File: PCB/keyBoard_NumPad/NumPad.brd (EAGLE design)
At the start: 88.9 x 142.9 mm, 174 parts, among them J1 J, J10 J, J11 J, J12 J, J13 J, J14 J, J15 J, J16 J, J17 J, J2 J, J3 J, J4 J, J5 J, J6 J, J7 J, J8 J, J9 J

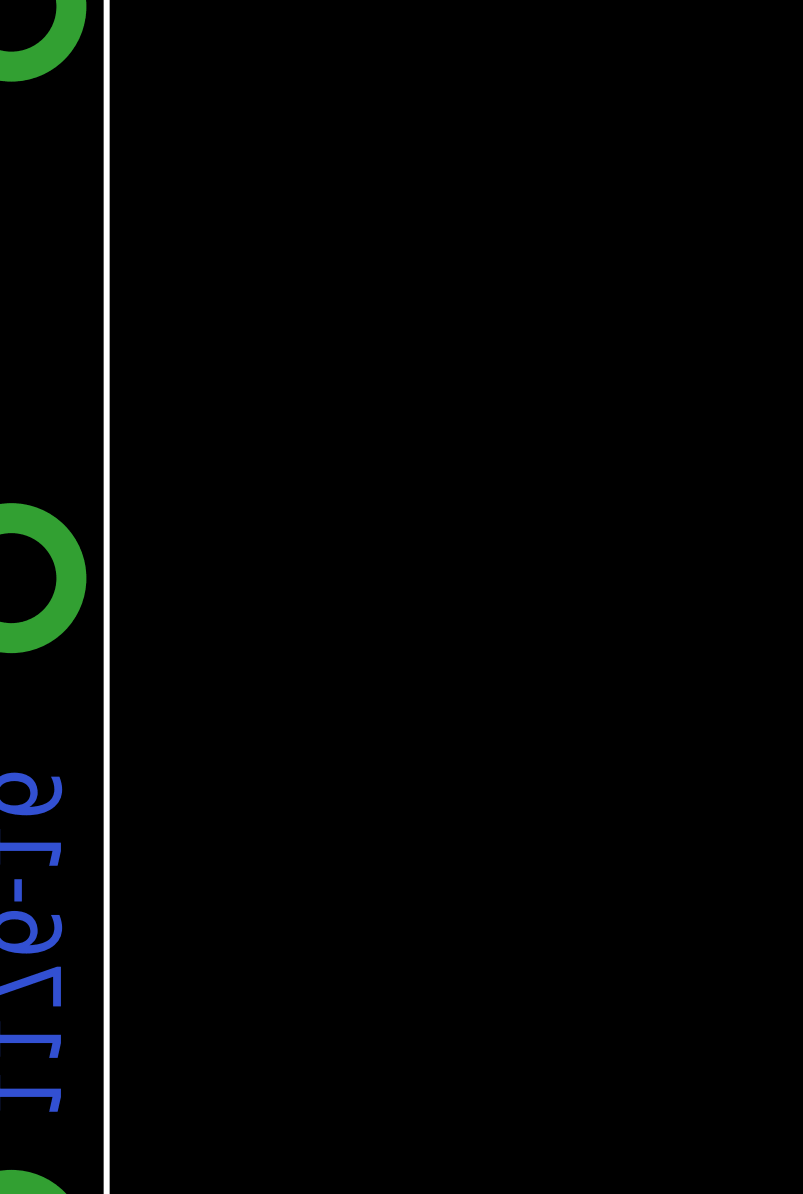
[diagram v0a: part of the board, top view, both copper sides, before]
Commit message: add1
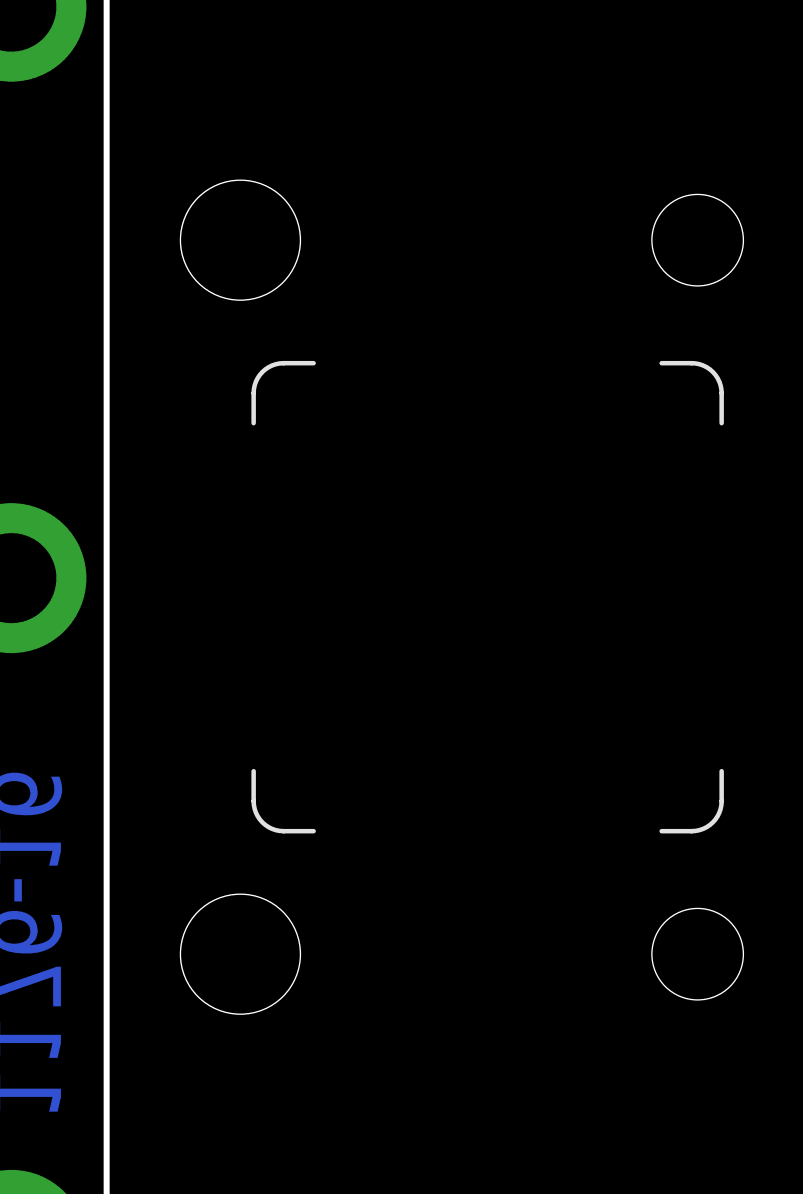
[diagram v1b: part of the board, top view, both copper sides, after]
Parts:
- added STAB_NEN: STAB, kbmxco:ZEALIOS-PCB_2U
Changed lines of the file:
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@@
 <?xml version="1.0" encoding="utf-8"?>
 <!DOCTYPE eagle SYSTEM "eagle.dtd">
-<eagle version="6.3">
+<eagle version="6.4">
 <drawing>
 <settings>
@@
 <circle x="43.4975" y="115.57" radius="3" width="0.254" layer="20"/>
 <circle x="62.5475" y="77.47" radius="3" width="0.254" layer="20"/>
-<dimension x1="18.0975" y1="156.36875" x2="106.9975" y2="154.94" x3="62.5475" y3="159.86125" layer="130" dtype="horizontal"/>
-<dimension x1="107.6325" y1="156.845" x2="106.68" y2="13.97" x3="117.7925" y3="85.4075" layer="130" dtype="vertical"/>
+<dimension x1="18.0975" y1="156.36875" x2="106.9975" y2="154.94" x3="62.5475" y3="159.86125" textsize="3.5" layer="130" dtype="horizontal"/>
+<dimension x1="107.6325" y1="156.845" x2="106.68" y2="13.97" x3="117.7925" y3="85.4075" textsize="3.5" layer="130" dtype="vertical"/>
 <wire x1="103.8225" y1="156.845" x2="21.2725" y2="156.845" width="0.2" layer="20"/>
-<dimension x1="108.74375" y1="115.57" x2="108.42625" y2="96.52" x3="113.82375" y3="106.045" layer="130" dtype="vertical"/>
+<dimension x1="108.74375" y1="115.57" x2="108.42625" y2="96.52" x3="113.82375" y3="106.045" textsize="3.5" layer="130" dtype="vertical"/>
 <wire x1="106.9975" y1="153.67" x2="106.9975" y2="17.145" width="0.2" layer="20"/>
 <wire x1="106.9975" y1="17.145" x2="103.8225" y2="13.97" width="0.2" layer="20" curve="-90"/>
@@
 <element name="U$24" library="kbmxco" package="KEY" value="" x="36.5125" y="125.095"/>
 <element name="U$26" library="kbmxco" package="SIZE132" value="" x="13.0175" y="88.5825"/>
+<element name="STAB_NEN" library="kbmxco" package="ZEALIOS-PCB_2U" value="STAB" x="119.6975" y="38.735" rot="R270"/>
 </elements>
 <signals>

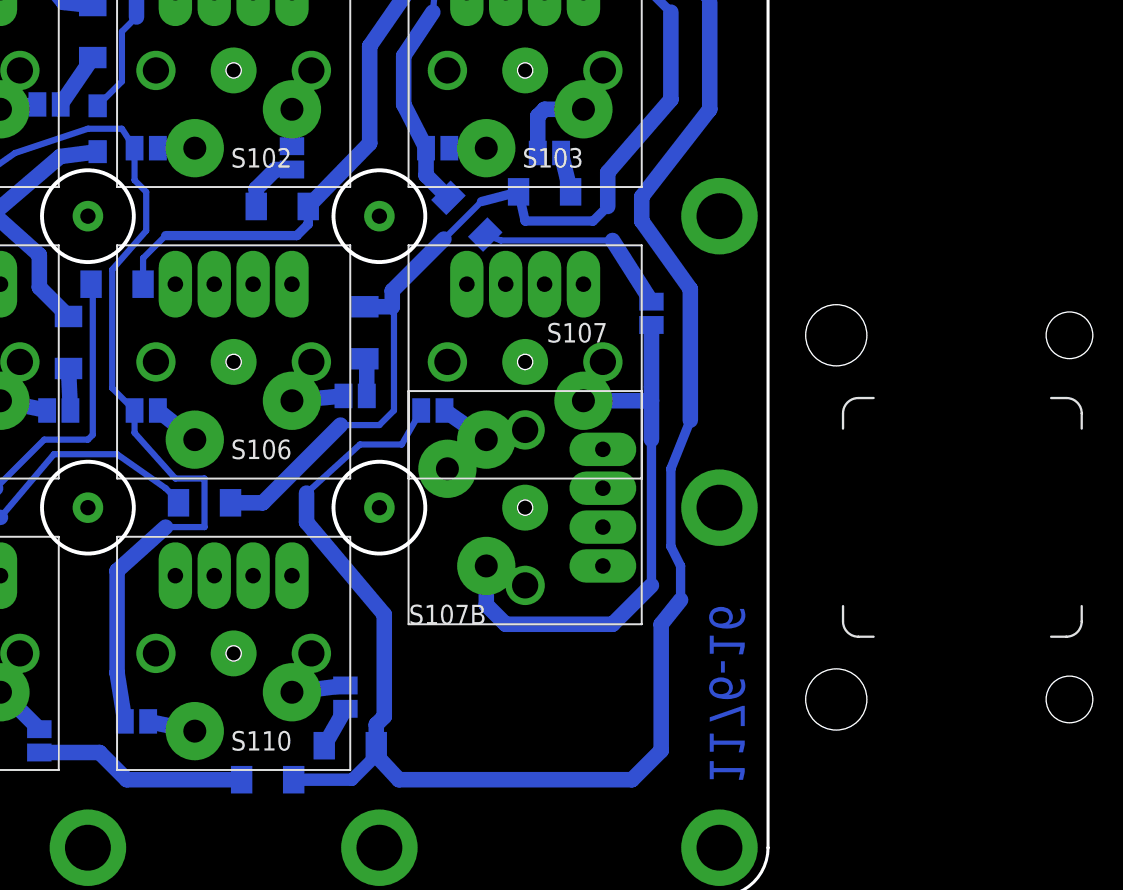
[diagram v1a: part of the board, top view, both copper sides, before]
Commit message: add2
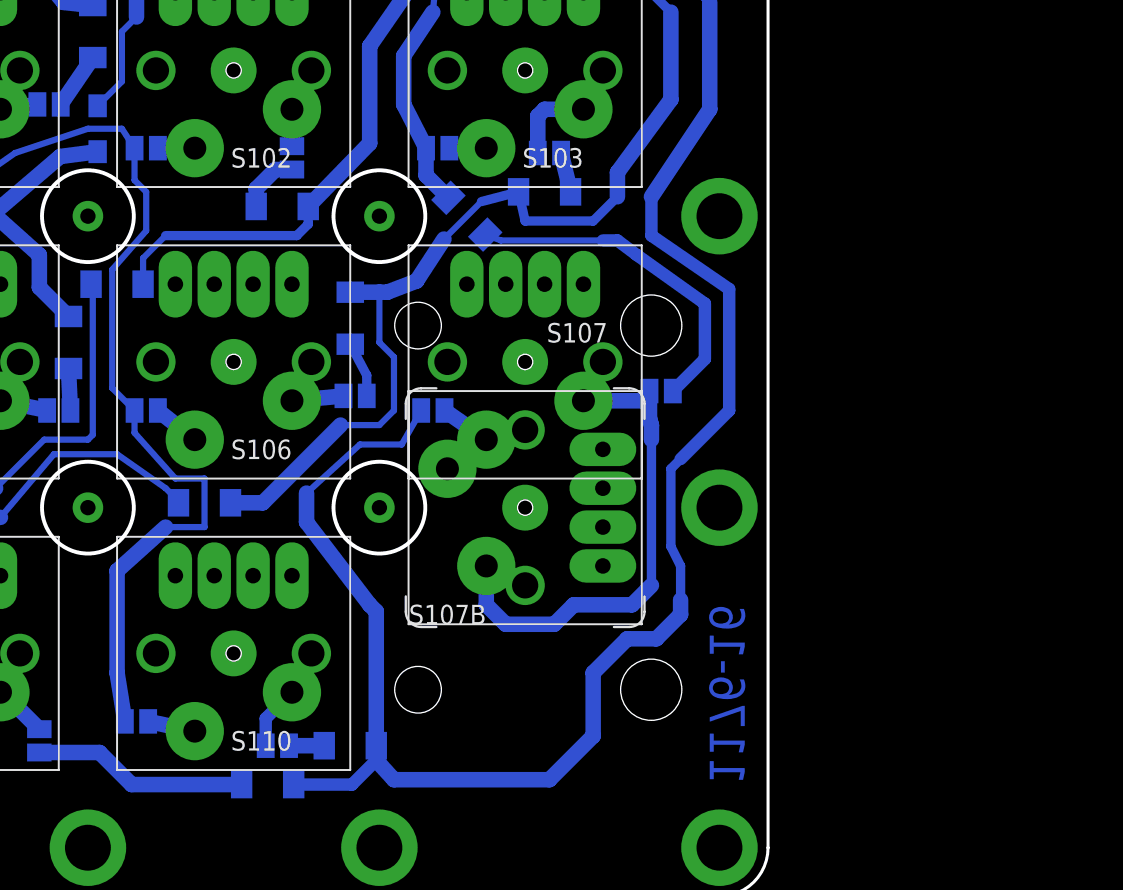
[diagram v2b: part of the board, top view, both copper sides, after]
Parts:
- moved STAB_NEN 28.6 mm to (91.1, 39.4), turned to 90 degrees
- moved JB110 5.46 mm to (74.9, 23.8), turned to 0 degrees
- moved JB107 5.12 mm to (100.0, 47.0), turned to 0 degrees
- moved D106 1.35 mm to (79.7, 51.8)
- moved D109 0.32 mm to (74.3, 21.3)
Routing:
- net N$3: track 13.1 -> 22.3 mm
- net N$319: track 36.4 -> 31.9 mm
- net N$36: track 132.8 -> 134.1 mm
- net N$325: track 2.48 -> 3.65 mm
- net N$336: track 3.52 -> 4.20 mm
